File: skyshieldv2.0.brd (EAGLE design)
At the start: 17.8 x 43.2 mm, 11 parts, among them J1 HEAD15-NOSS, J2 HEAD15-NOSS-1

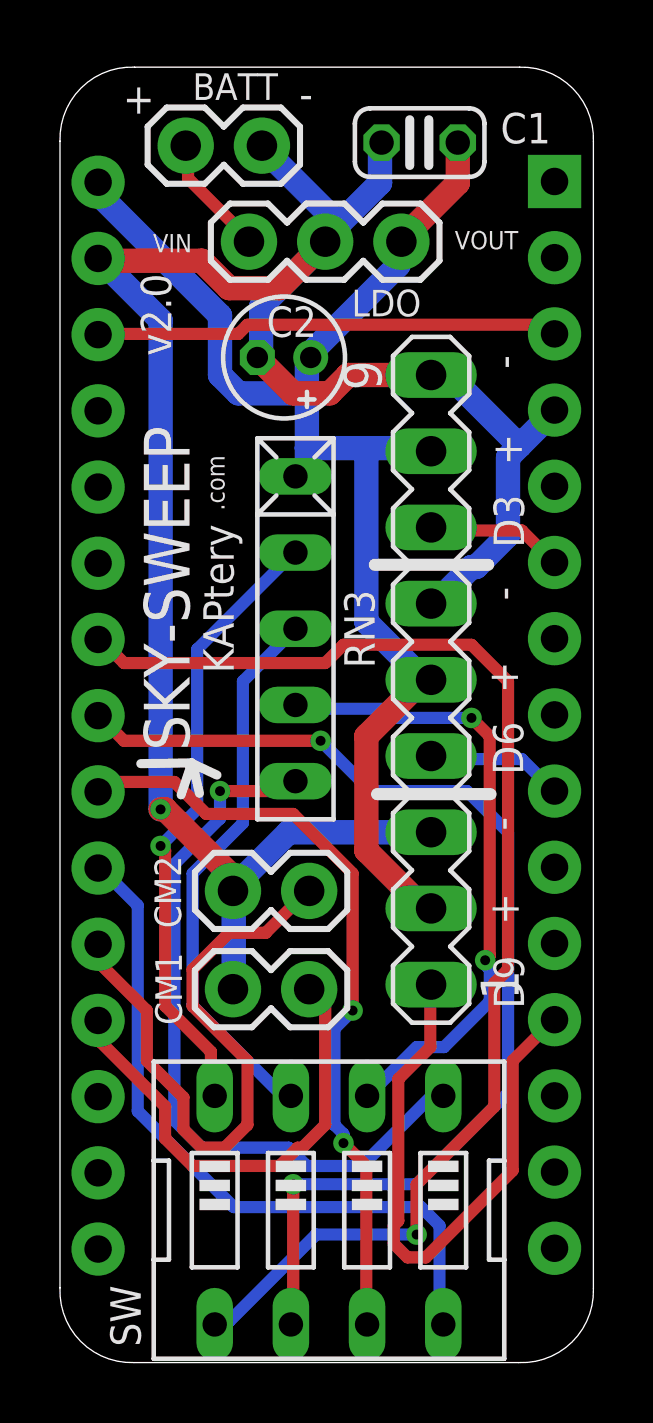
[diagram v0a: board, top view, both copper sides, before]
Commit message: update
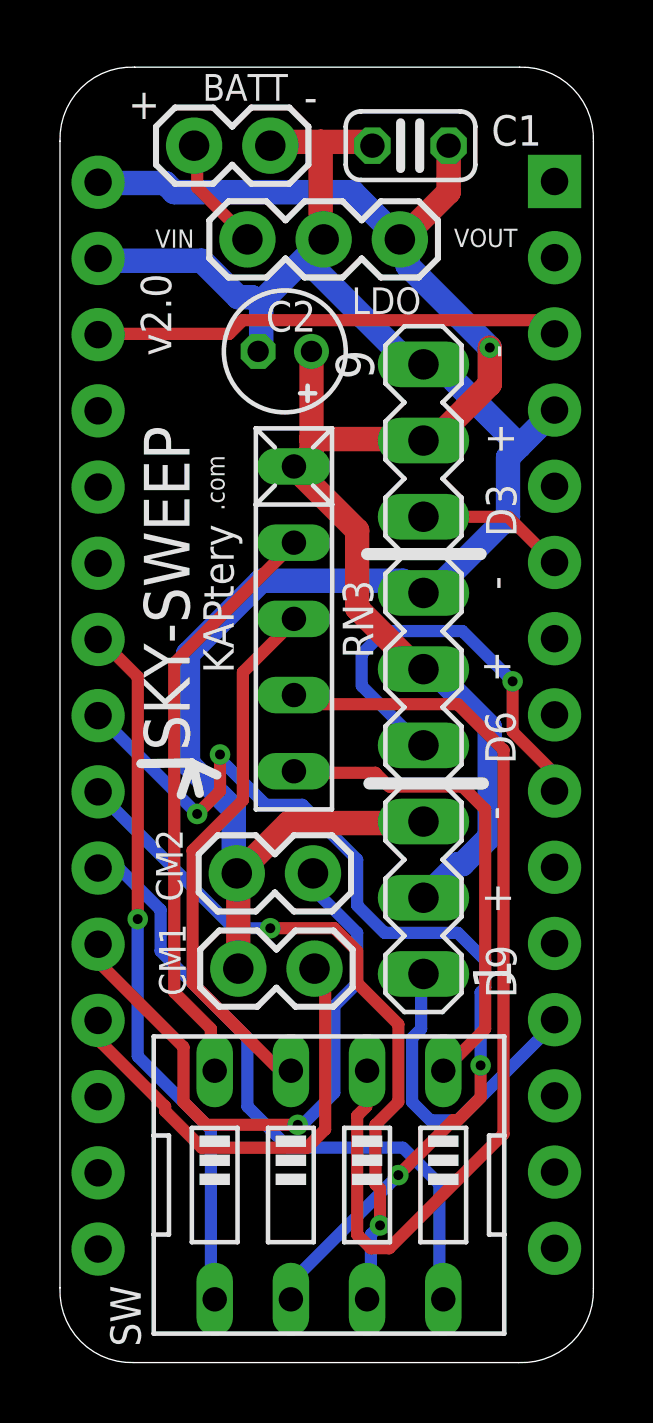
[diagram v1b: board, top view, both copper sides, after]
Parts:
- moved SW1 0.84 mm to (8.97, 5.92)
- moved CHDKA 0.71 mm to (5.94, 13.1)
- moved CHDKB 0.60 mm to (5.89, 16.3)
- moved SV4 0.44 mm to (12.1, 23.1)
- moved RN3 0.33 mm to (7.80, 24.8)
- moved C1 0.32 mm to (11.7, 40.6)
- moved BATT 0.28 mm to (4.47, 40.6)
- moved C2 0.20 mm to (7.49, 33.7)
- moved LDO-5V 0.09 mm to (11.3, 37.4)
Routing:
- net A5: track 42.5 -> 23.7 mm
- net N$8: track 21.3 -> 32.8 mm, vias 2 -> 0
- net GND: track 74.4 -> 63.2 mm, vias 1 -> 0
- net D6: track 4.59 -> 14.2 mm, vias 0 -> 1
- net D9: track 20.1 -> 11.1 mm
- net N$9: track 24.8 -> 16.2 mm, vias 1 -> 0
- net A4: track 37.1 -> 33.7 mm, vias 2 -> 4
- net VCC: track 47.4 -> 50.1 mm, vias 0 -> 1
- net A3: track 25.6 -> 23.6 mm
- net A2: track 23.7 -> 21.8 mm
- net N$5: track 20.8 -> 19.9 mm, vias 1 -> 0
- net N$7: track 18.5 -> 18.0 mm
- net A1: track 21.0 -> 20.5 mm, vias 0 -> 1
